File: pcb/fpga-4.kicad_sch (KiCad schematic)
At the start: 4 parts, among them U5 XC7A100T-FGG484

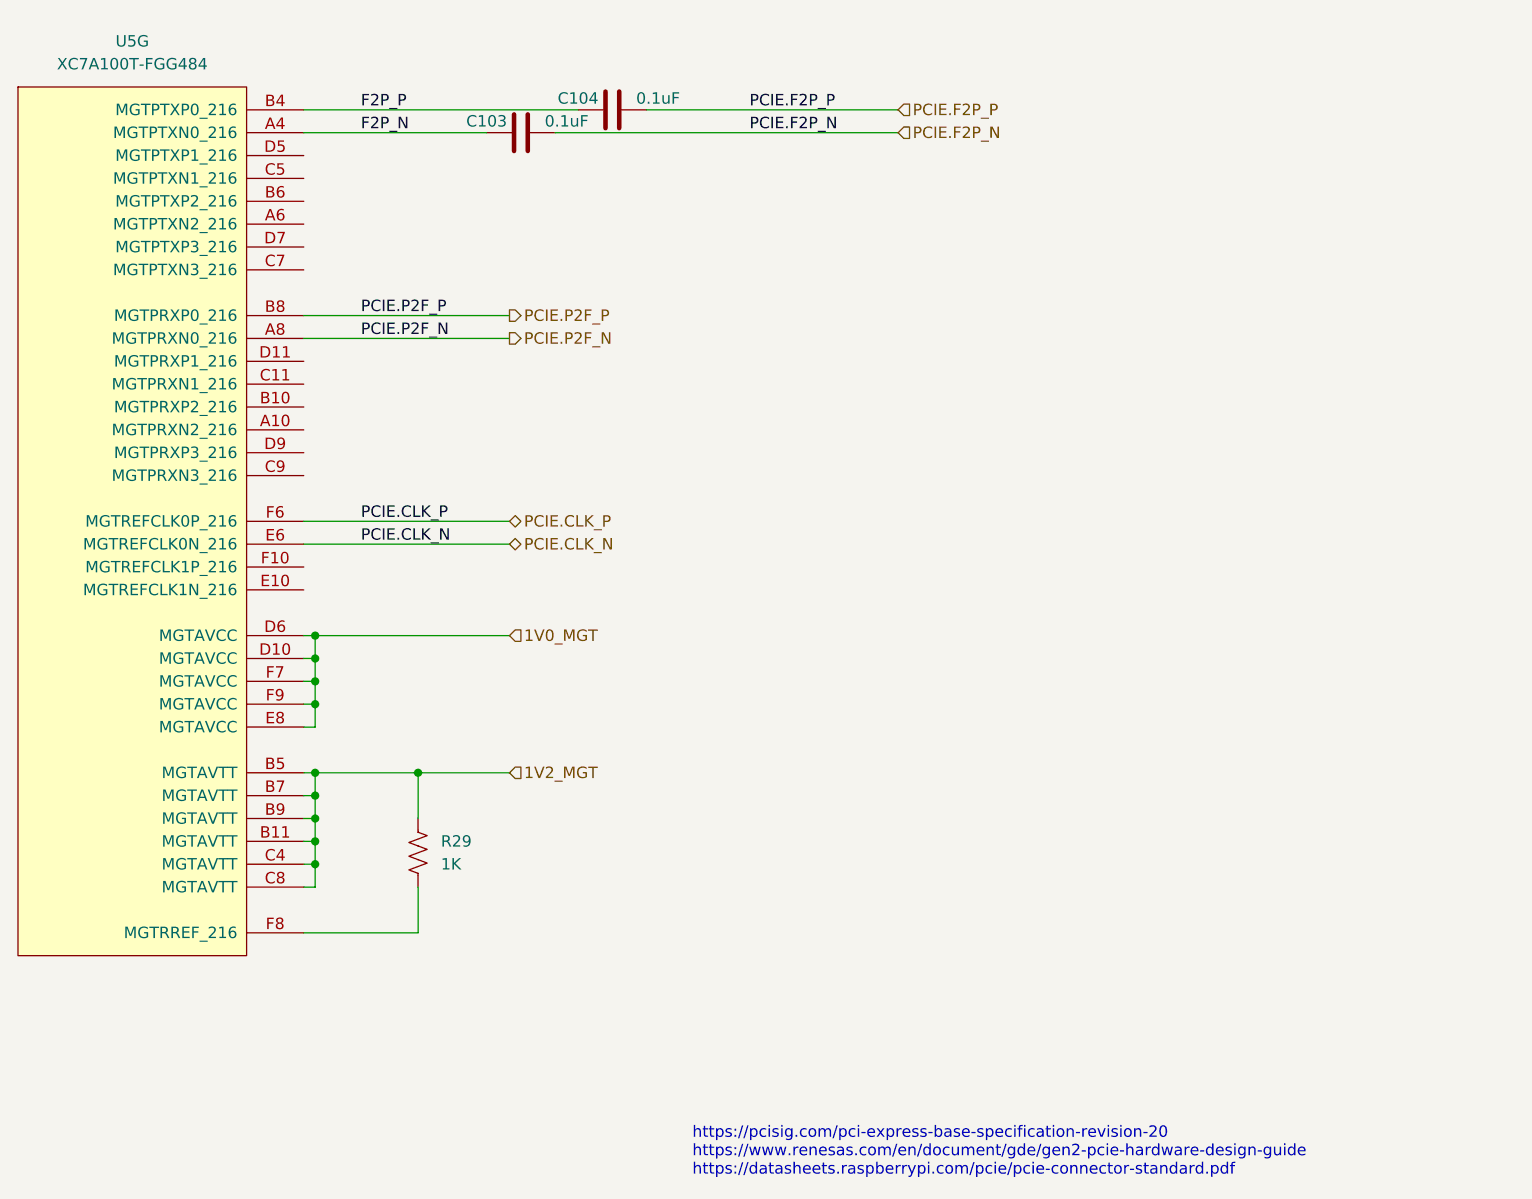
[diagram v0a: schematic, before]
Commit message: power restructuring
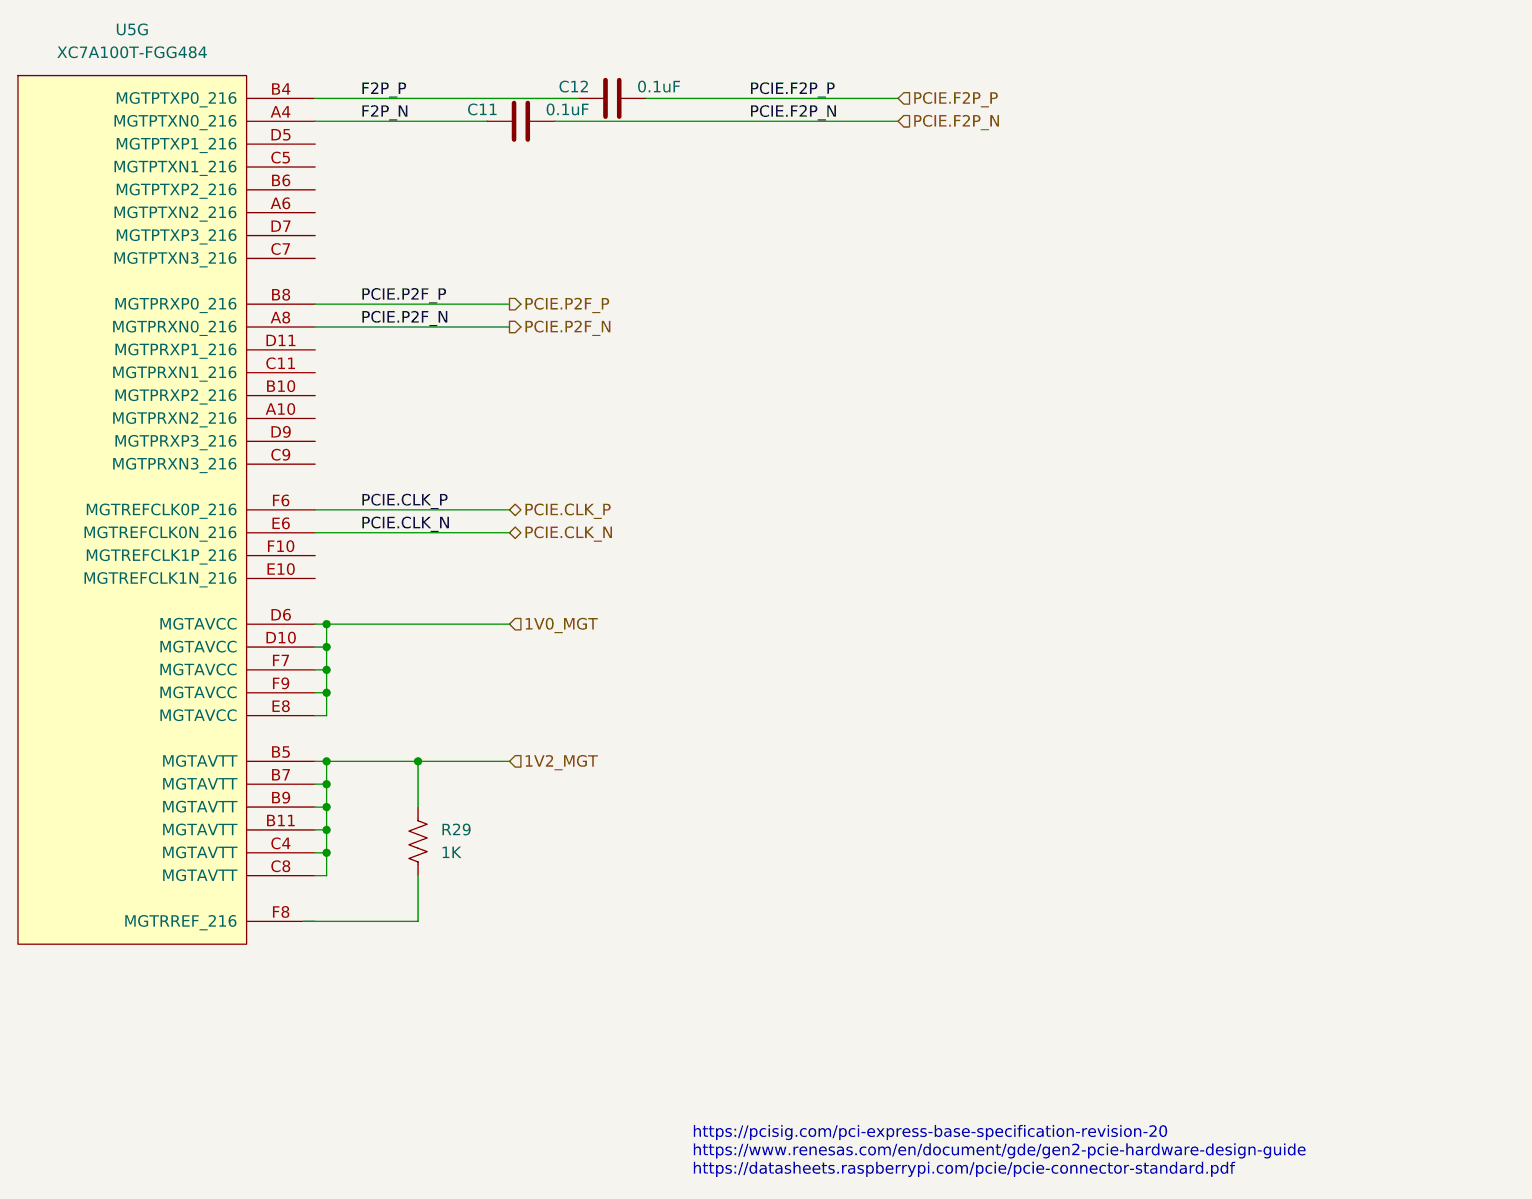
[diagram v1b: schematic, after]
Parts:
- removed C103, C104: 0.1uF, Capacitor_SMD:C_0402_1005Metric, symbol library:C
- added C11, C12: 0.1uF, Capacitor_SMD:C_0402_1005Metric, symbol library:C
- U5: symbol FPGA_Xilinx_Artix7:XC7A100T-FGG484 -> library:XC7A100T-FGG484
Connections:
- net F2P_N: now also C11.1
- net F2P_P: now also C12.1
- net PCIE.F2P_N: now also C11.2
- net PCIE.F2P_P: now also C12.2
- net at U5.F8 (MGTRREF_216): no longer R29.1
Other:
- moved on the sheet: R29, U5G
